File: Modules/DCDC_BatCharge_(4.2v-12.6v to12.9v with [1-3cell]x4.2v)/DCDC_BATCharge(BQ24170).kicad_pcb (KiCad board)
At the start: 2 copper layers, 44 x 44 mm, 88 parts, among them J1 Btn_LED, J2 VIA_V_BAT, J3 VIA_GND, J4 VIA_V_Adapter, J5 VIA_V_SYS, Q1 AO3416, Q2 AO3416, Q3 AO3415, U1 BQ24170, U2 TPS61288, U3 TPS61288

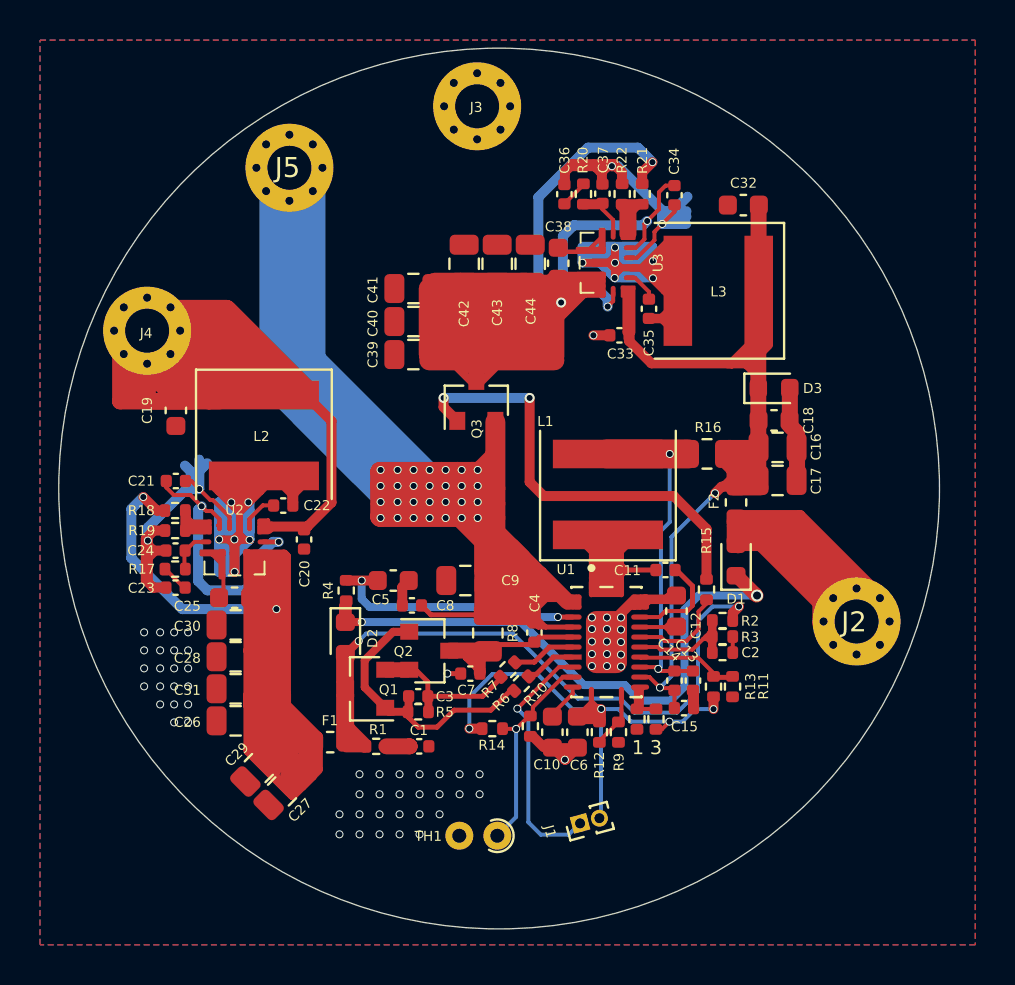
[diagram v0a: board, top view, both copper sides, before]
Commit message: update modules
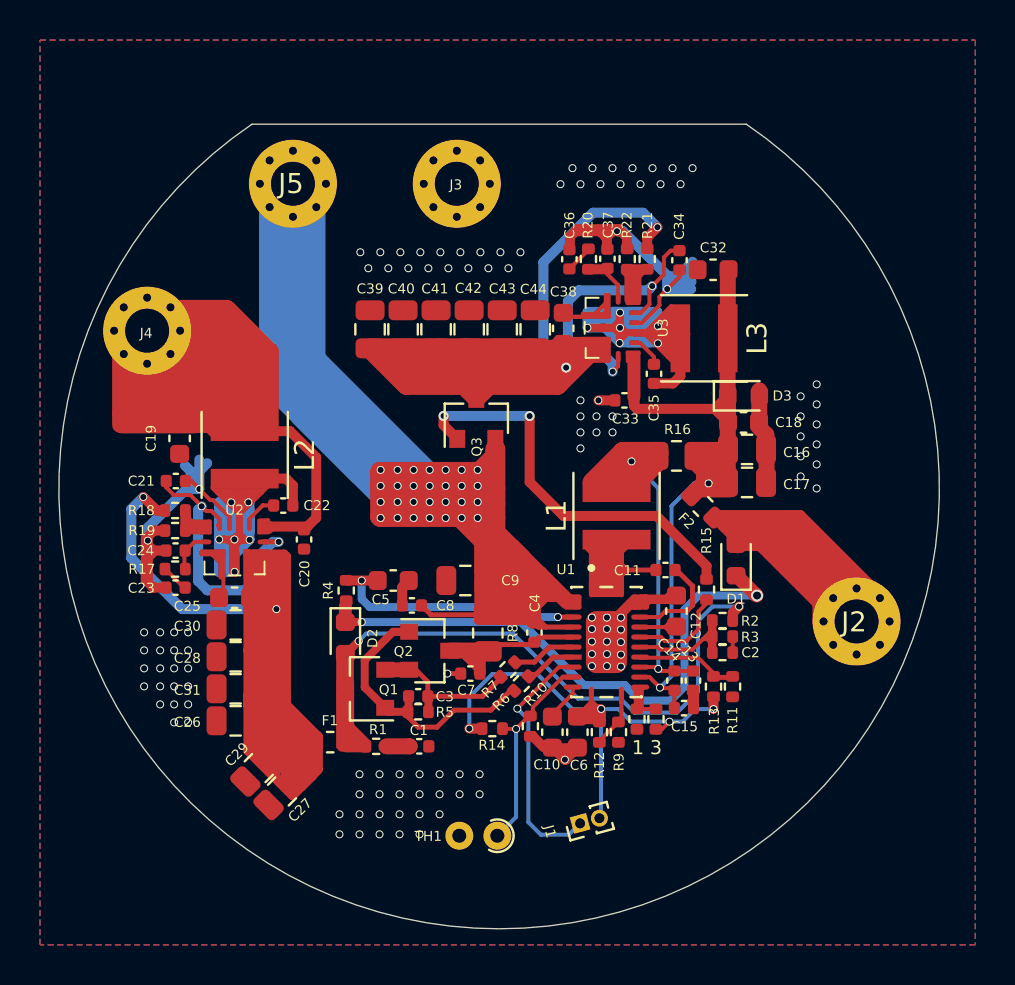
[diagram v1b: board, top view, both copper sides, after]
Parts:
- F1: value 4A -> 3.5A
- L1: value 3.3uH CoilCraft 6030 -> 3.3uH CoilCraft 40xx; footprint Inductor_SMD:L_Coilcraft_XAL60xx_6.36x6.56mm -> Inductor_SMD:L_Coilcraft_XxL4020
- L2, L3: value 1.8uH CoilCraft 6030 -> 1.8uH CoilCraft 40xx; footprint Inductor_SMD:L_Coilcraft_XAL60xx_6.36x6.56mm -> Inductor_SMD:L_Coilcraft_XxL4020
- R20: value 41.2k -> 47.5k
- moved J3 4.00 mm to (148.1, 73.3)
- moved C32 3.57 mm to (160.9, 77.6)
- moved C42 3.28 mm to (148.7, 80.6)
- moved C43 3.28 mm to (150.3, 80.6)
- moved C44 3.28 mm to (152.0, 80.6)
- moved C33 3.26 mm to (156.4, 84.1)
- moved C34 3.26 mm to (159.2, 77.1)
- moved C35 3.26 mm to (157.9, 82.8)
- moved C36 3.26 mm to (153.7, 77.1)
- moved C37 3.26 mm to (155.6, 77.0)
- moved C38 3.26 mm to (153.4, 80.5)
- moved R20 3.26 mm to (154.6, 77.0)
- moved R21 3.26 mm to (157.6, 77.0)
- moved R22 3.26 mm to (156.6, 77.0)
- moved U3 3.26 mm to (155.7, 80.5)
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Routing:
- net Adapter: track 100.8 -> 125.0 mm
- net V_BAT_OUT: track 54.2 -> 46.6 mm
- net V_BAT: track 64.8 -> 68.3 mm
- net Net-(C13-Pad2): track 22.0 -> 24.0 mm
- net Net-(Q3-Pad1): track 22.3 -> 20.3 mm
- net V_BAT_BOOST: track 76.4 -> 77.9 mm
- net GND: vias 68 -> 118
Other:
- board size 44 x 44 mm -> 44 x 40.2 mm
